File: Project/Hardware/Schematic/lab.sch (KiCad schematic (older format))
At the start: 29 parts, among them J1 USB_B_Micro, J2 6P Male, J3 Conn_01x03_Male, U1 NCP1117-5.0_SOT223, U2 STM32F411RETx, U3 NCP1117-3.3_SOT223, Y1 8MHz

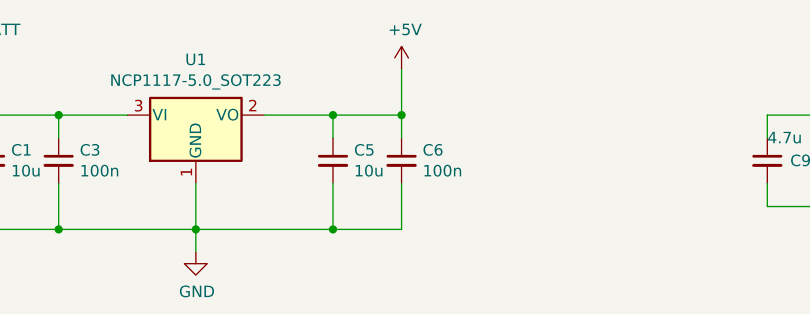
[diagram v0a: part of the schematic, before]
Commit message: Ny display, igen!
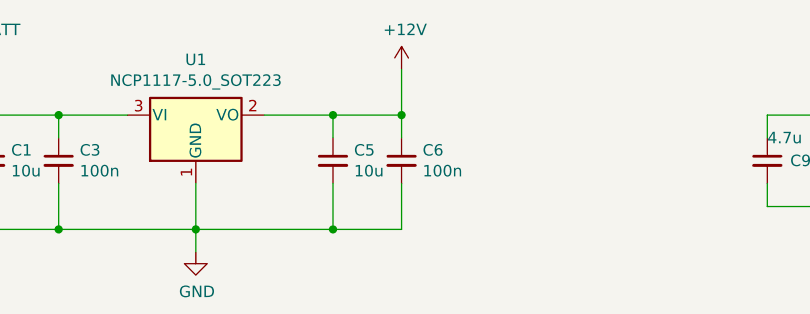
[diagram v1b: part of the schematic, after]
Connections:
- net +5V: no longer C5.1, C6.1, U1.2 (VO)
- new net +12V: C5.1, C6.1, U1.2 (VO)
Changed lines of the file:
@@
 	3600 1100 3900 1100
 Connection ~ 3900 1100
-$Comp
-L power:+5V #PWR0112
-U 1 1 5C5E5791
-P 4200 900
-F 0 "#PWR0112" H 4200 750 50  0001 C CNN
-F 1 "+5V" H 4215 1073 50  0000 C CNN
-F 2 "" H 4200 900 50  0001 C CNN
-F 3 "" H 4200 900 50  0001 C CNN
-	1    4200 900
-	1    0    0    -1
-$EndComp
 Wire Wire Line
 	3900 1600 3300 1600
@@
 Wire Wire Line
 	9250 5200 9650 5200
+$Comp
+L power:+12V #PWR?
+U 1 1 5C679F70
+P 4200 900
+F 0 "#PWR?" H 4200 750 50  0001 C CNN
+F 1 "+12V" H 4215 1073 50  0000 C CNN
+F 2 "" H 4200 900 50  0001 C CNN
+F 3 "" H 4200 900 50  0001 C CNN
+	1    4200 900
+	1    0    0    -1
+$EndComp
 $EndSCHEMATC
